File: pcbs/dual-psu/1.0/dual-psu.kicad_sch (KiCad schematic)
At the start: 97 parts, among them J1 Conn_01x02_Pin, J10 Conn_01x03_Male, J11 Conn_01x03_Male, J12 Conn_01x02_Pin, J13 Conn_01x02_Pin, J14 Conn_01x03_Male, J15 Conn_01x03_Male, J16 Conn_01x02_Pin, J17 Conn_01x02_Pin, J18 Conn_01x02_Male, J19 Conn_01x03_Male, J2 Conn_01x02_Pin, J20 Conn_01x03_Male, J21 Conn_01x03_Male, J22 Conn_01x03_Male, J23 Conn_01x02_Pin, J24 Conn_01x02_Pin, J25 Conn_01x02_Pin, J26 Conn_01x02_Pin, J27 Conn_01x03_Male, J28 Conn_01x02_Pin, J3 Conn_01x03_Male, J4 Conn_01x03_Male, J5 Conn_01x03_Male, J6 Conn_01x03_Male, J7 Conn_01x02_Pin, J8 Conn_01x02_Pin, J9 Conn_01x03_Pin, U1 AMS1117-5.0, U10 INA260, U11 TMP100, U12 NCP1117-12, U13 AP64351SP-13, U2 AMS1117-5.0, U3 ZLDO1117QG33TA, U4 ZLDO1117QG33TA, U5 LM317_SOT-223, U6 LM337_SOT223, U7 INA260, U8 INA260, U9 INA260

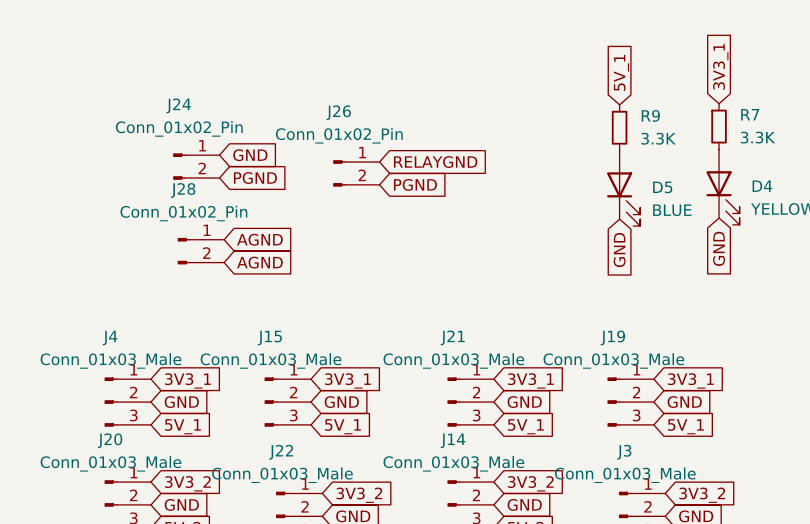
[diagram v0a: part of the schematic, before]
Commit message: Updating readmes
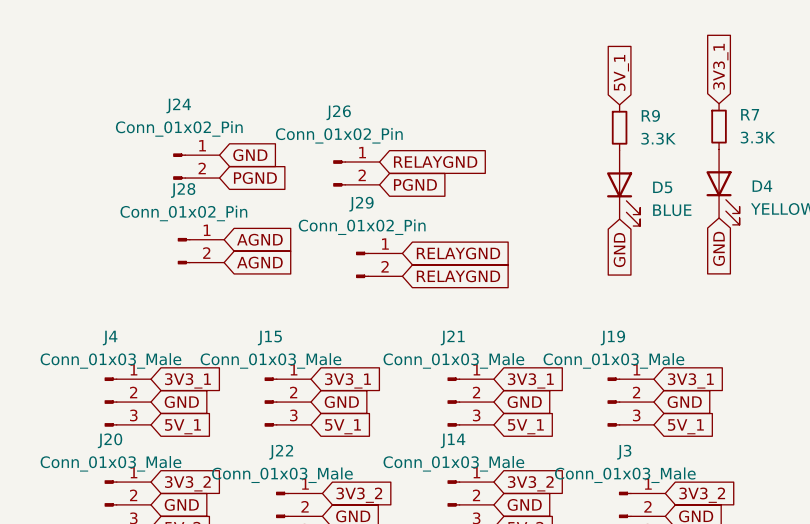
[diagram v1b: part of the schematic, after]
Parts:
- added J29: Conn_01x02_Pin, Connector_JST:JST_PH_B2B-PH-K_1x02_P2.00mm_Vertical, symbol Connector:Conn_01x02_Pin
- D1, D2, D7: footprint LED_SMD:LED_0805_2012Metric_Pad1.15x1.40mm_HandSolder -> LED_SMD:LED_0603_1608Metric
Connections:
- net RELAYGND: now also J29.1 (Pin_1), J29.2 (Pin_2)
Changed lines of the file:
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@@
 		)
 	)
+	(global_label "RELAYGND"
+		(shape input)
+		(at 262.89 44.45 0)
+		(fields_autoplaced yes)
+		(effects
+			(font
+				(size 1.27 1.27)
+			)
+			(justify left)
+		)
+		(property "Intersheetrefs" "${INTERSHEET_REFS}"
+			(at 275.37 44.45 0)
+			(effects
+				(font
+					(size 1.27 1.27)
+				)
+				(justify left)
+				(hide yes)
+			)
+		)
+	)
 	(global_label "3V3_1"
 		(shape input)
@@
 		)
 	)
+	(global_label "RELAYGND"
+		(shape input)
+		(at 262.89 41.91 0)
+		(fields_autoplaced yes)
+		(effects
+			(font
+				(size 1.27 1.27)
+			)
+			(justify left)
+		)
+		(property "Intersheetrefs" "${INTERSHEET_REFS}"
+			(at 275.37 41.91 0)
+			(effects
+				(font
+					(size 1.27 1.27)
+				)
+				(justify left)
+				(hide yes)
+			)
+		)
+	)
 	(global_label "3V3_1"
 		(shape input)
@@
 			)
 		)
-		(property "Footprint" "LED_SMD:LED_0805_2012Metric_Pad1.15x1.40mm_HandSolder"
+		(property "Footprint" "LED_SMD:LED_0603_1608Metric"
 			(at 367.919 44.323 0)
 			(effects
@@
 	)
 	(symbol
+		(lib_id "Connector:Conn_01x02_Pin")
+		(at 257.81 41.91 0)
+		(unit 1)
+		(exclude_from_sim no)
+		(in_bom yes)
+		(on_board yes)
+		(dnp no)
+		(fields_autoplaced yes)
+		(property "Reference" "J29"
+			(at 258.445 36.322 0)
+			(effects
+				(font
+					(size 1.27 1.27)
+				)
+			)
+		)
+		(property "Value" "Conn_01x02_Pin"
+			(at 258.445 38.862 0)
+			(effects
+				(font
+					(size 1.27 1.27)
+				)
+			)
+		)
+		(property "Footprint" "Connector_JST:JST_PH_B2B-PH-K_1x02_P2.00mm_Vertical"
+			(at 257.81 41.91 0)
+			(effects
+				(font
+					(size 1.27 1.27)
+				)
+				(hide yes)
+			)
+		)
+		(property "Datasheet" "~"
+			(at 257.81 41.91 0)
+			(effects
+				(font
+					(size 1.27 1.27)
+				)
+				(hide yes)
+			)
+		)
+		(property "Description" ""
+			(at 257.81 41.91 0)
+			(effects
+				(font
+					(size 1.27 1.27)
+				)
+				(hide yes)
+			)
+		)
+		(pin "1"
+		)
+		(pin "2"
+		)
+		(instances
+			(project "dual-psu"
+				(path "/5486715c-d46c-4c73-9a76-76411783f9bd"
+					(reference "J29")
+					(unit 1)
+				)
+			)
+		)
+	)
+	(symbol
 		(lib_id "Device:C_Polarized_Small")
 		(at 162.56 147.32 0)
@@
 			)
 		)
-		(property "Footprint" "LED_SMD:LED_0805_2012Metric_Pad1.15x1.40mm_HandSolder"
+		(property "Footprint" "LED_SMD:LED_0603_1608Metric"
 			(at 382.27 46.99 0)
 			(effects
@@
 			)
 		)
-		(property "Footprint" "LED_SMD:LED_0805_2012Metric_Pad1.15x1.40mm_HandSolder"
+		(property "Footprint" "LED_SMD:LED_0603_1608Metric"
 			(at 354.33 46.99 0)
 			(effects

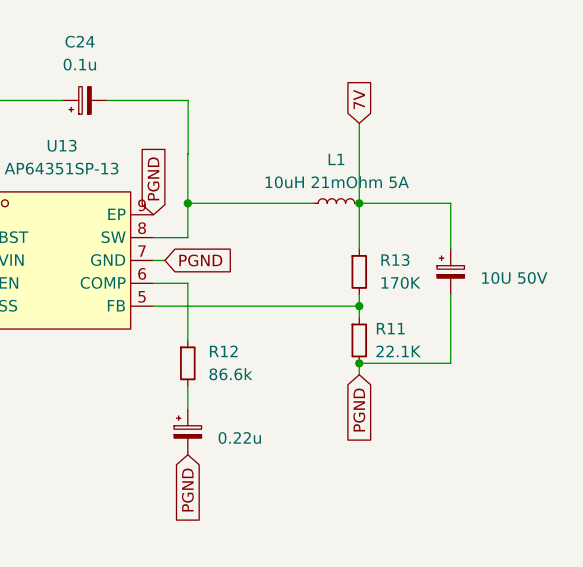
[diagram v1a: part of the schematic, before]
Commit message: Updates to pcbs
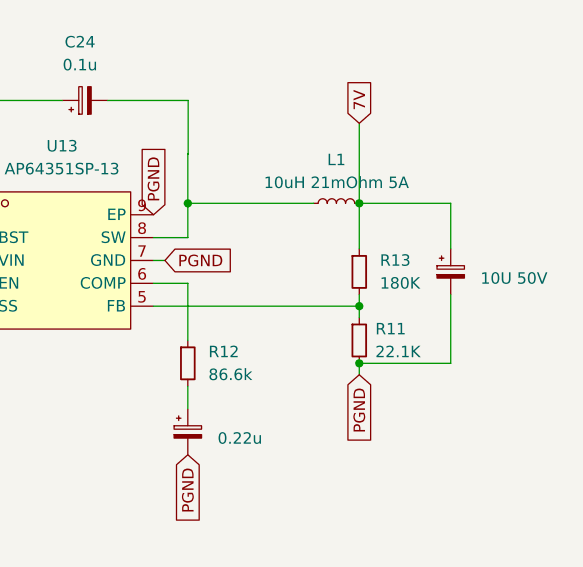
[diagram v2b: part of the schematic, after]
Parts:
- R13: value 170K -> 180K; Mouser (none) -> 603-RC0603JR-10180KL
- U13: Mouser (none) -> 621-AP64351SP-13
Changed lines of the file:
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@@
 			)
 		)
-		(property "Value" "170K"
+		(property "Value" "180K"
 			(at 373.126 121.9199 0)
 			(effects
@@
 			)
 		)
+		(property "Mouser" " 603-RC0603JR-10180KL "
+			(at 370.84 120.65 0)
+			(effects
+				(font
+					(size 1.27 1.27)
+				)
+				(hide yes)
+			)
+		)
 		(pin "1"
 		)
@@
 			(effects
 				(font
+					(size 1.27 1.27)
+				)
+				(hide yes)
+			)
+		)
+		(property "Mouser" " 621-AP64351SP-13 "
+			(at 337.82 119.38 0)
+			(effects
+				(font
